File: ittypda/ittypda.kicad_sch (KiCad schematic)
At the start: 147 parts, among them CN1 S2B-PH-SM4-TB, J1 USB_C_Receptacle_USB2.0_14P, SW1 SW_SPDT, U1 STM32F401RETx, U2 BQ24040DSQR, U3 TLV75801PDRV, Y1 16Mhz

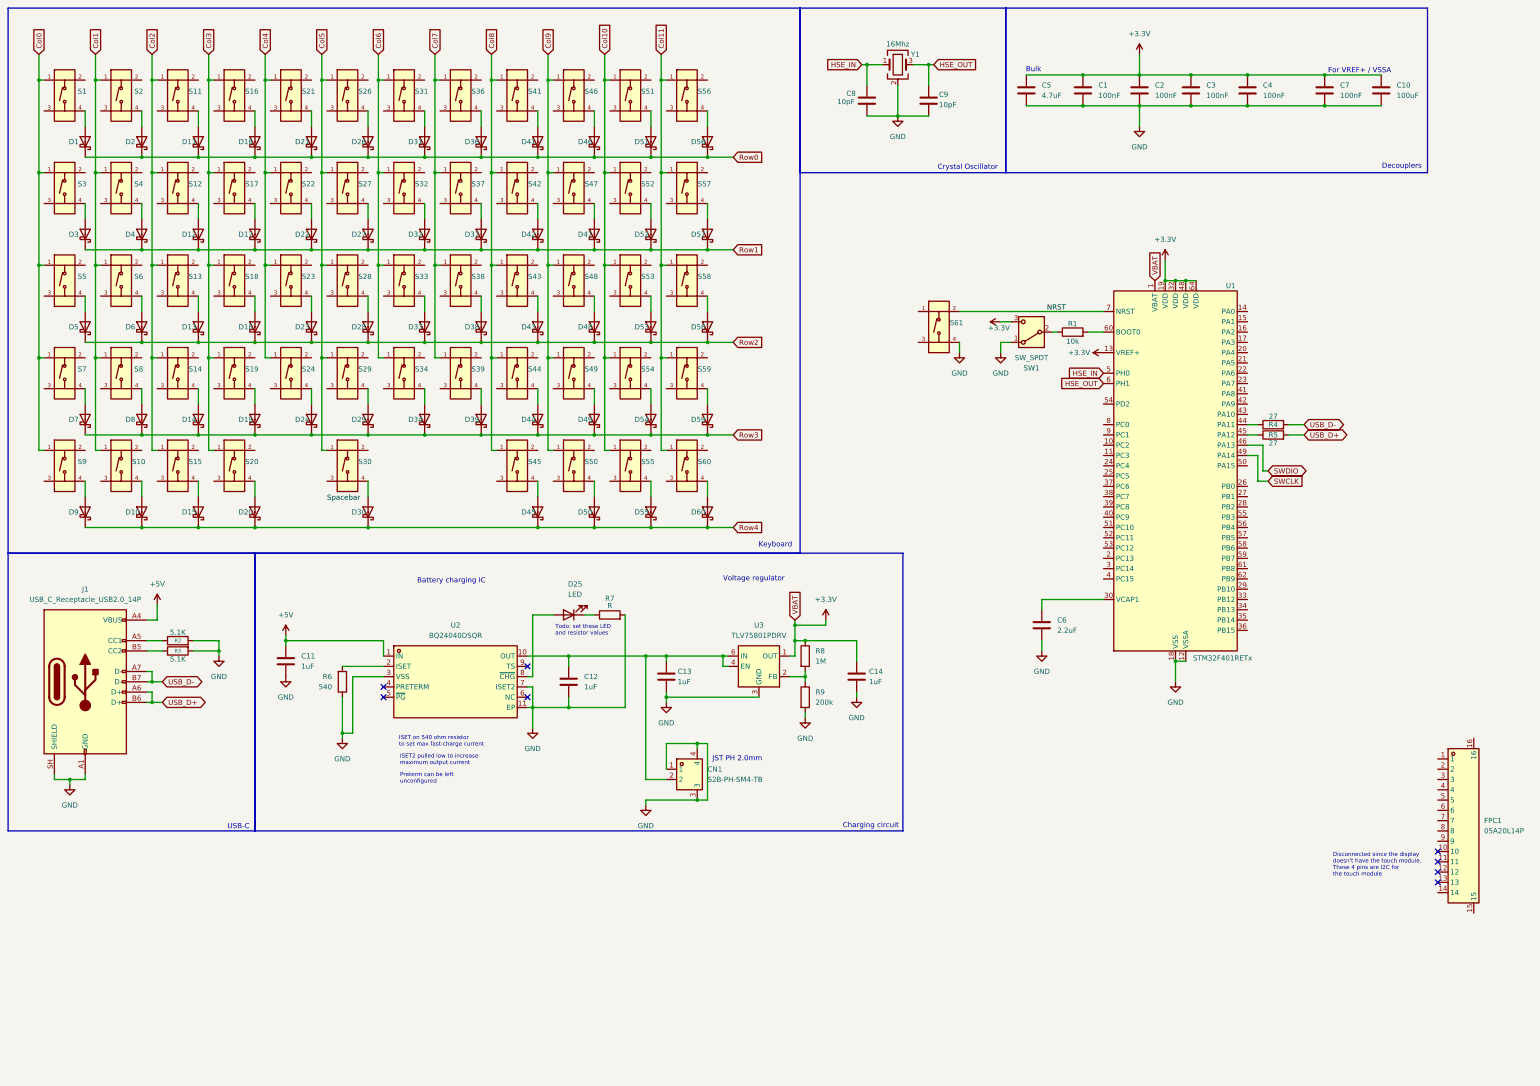
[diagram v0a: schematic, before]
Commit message: organize schem
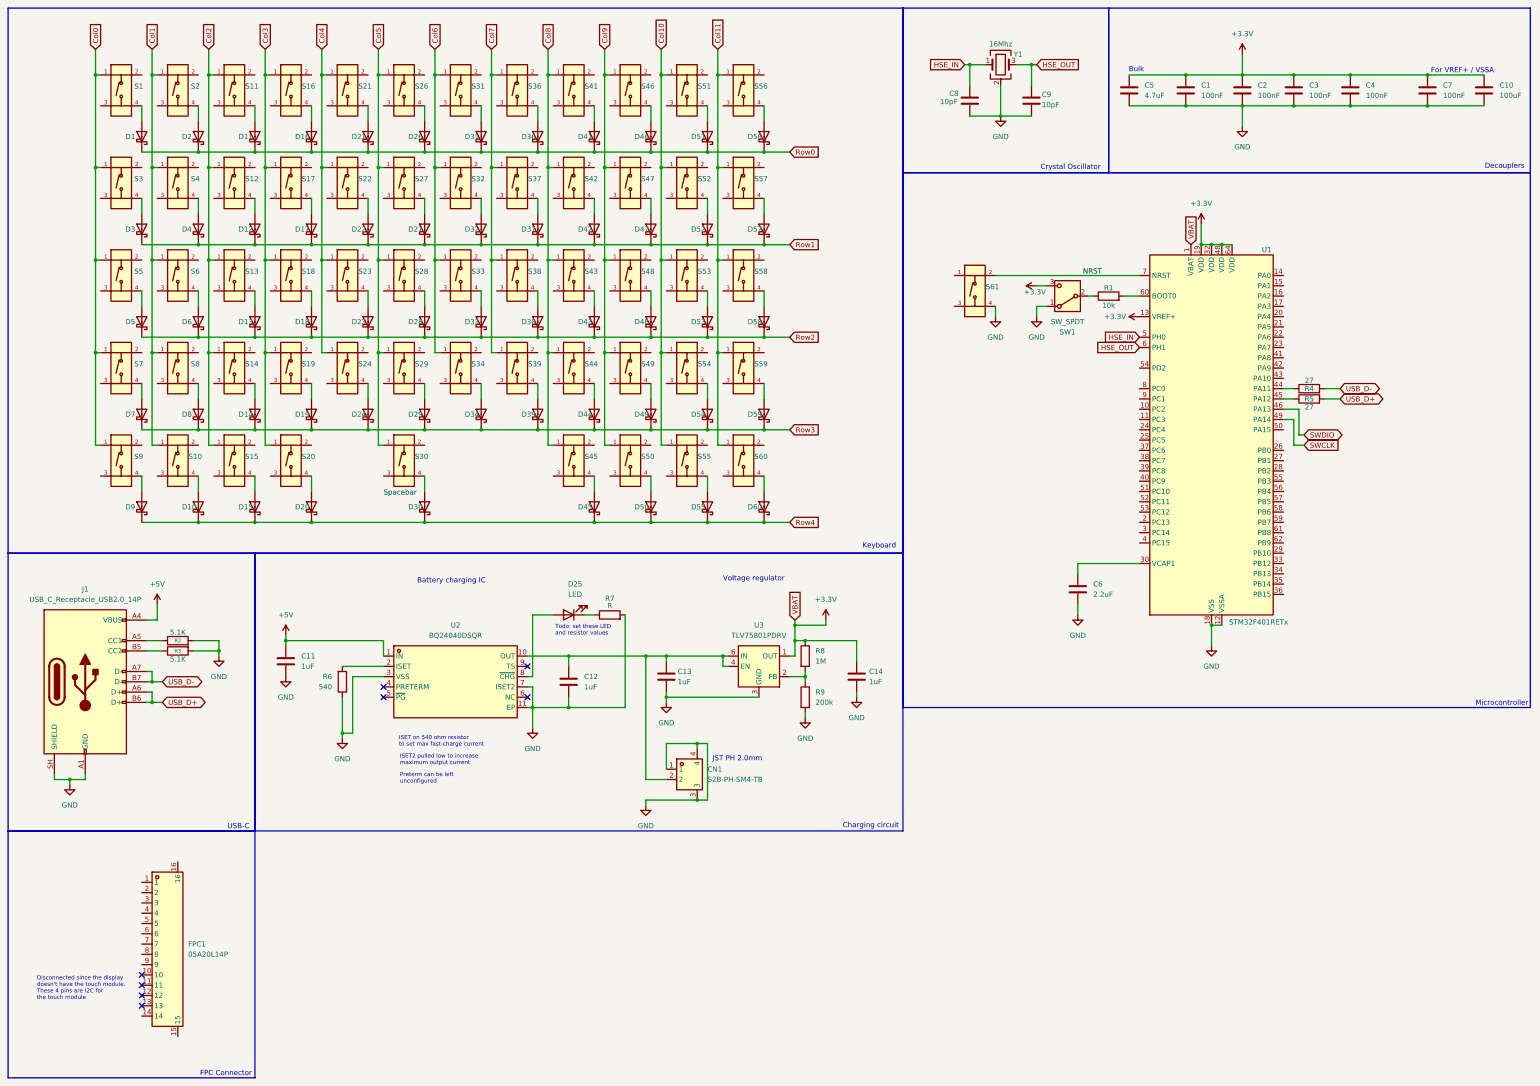
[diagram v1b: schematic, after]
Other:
- note added: "FPC Connector"
- note added: "Microcontroller"
- moved on the sheet: C1, C10, C2, C3, C4, C5, C6, C7, C8, C9, D1, D10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
